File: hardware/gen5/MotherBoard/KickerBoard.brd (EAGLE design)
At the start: 141.6 x 141.1 mm, 154 parts, among them U1 SAM3S4B

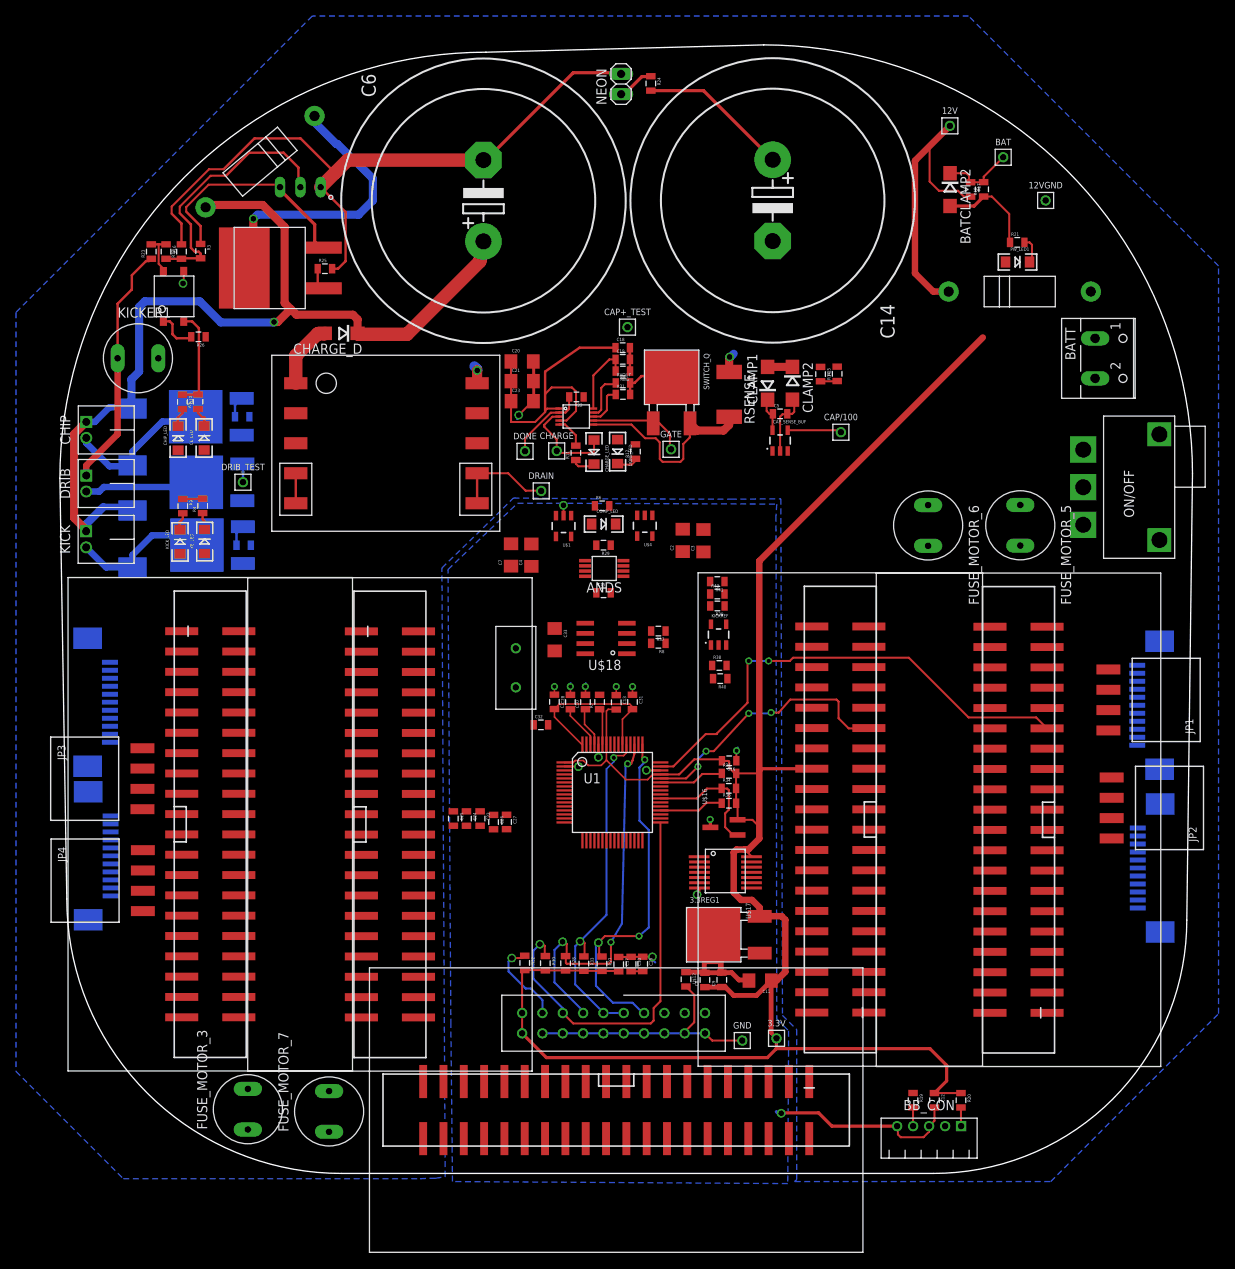
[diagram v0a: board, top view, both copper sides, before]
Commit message: More motherboard work!
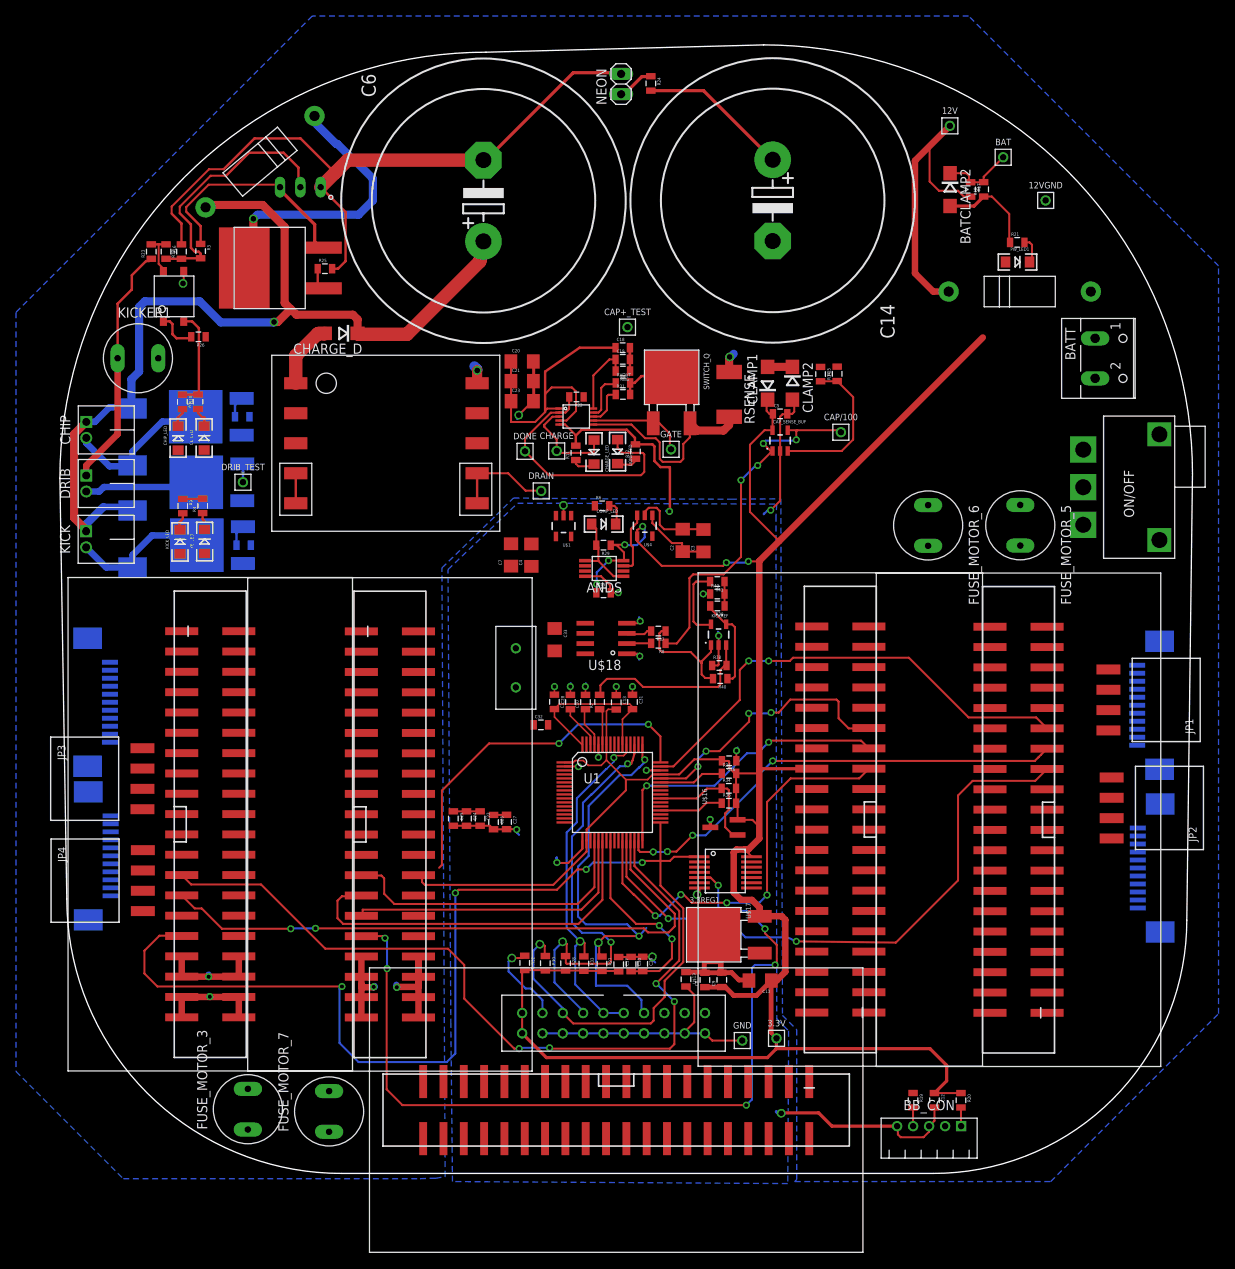
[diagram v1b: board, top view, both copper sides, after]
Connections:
- removed net N$39: MOTOR2.15, MOTOR2.16, MOTOR2.17, MOTOR2.18, U$8.6, U$8.7
- net 12VGND: now also MOTOR1.22, MOTOR1.33, MOTOR1.34, MOTOR2.15, MOTOR2.16, MOTOR2.17, MOTOR2.18, MOTOR2.22, MOTOR2.33, MOTOR2.34, MOTOR3.22, MOTOR3.33, MOTOR3.34, MOTOR4.22, MOTOR4.33, MOTOR4.34, U$10.5, U$11.5, U$8.6, U$8.7, U$9.5
- net GND: no longer MOTOR1.22, MOTOR1.33, MOTOR1.34, MOTOR2.22, MOTOR2.33, MOTOR2.34, MOTOR3.22, MOTOR3.33, MOTOR3.34, MOTOR4.22, MOTOR4.33, MOTOR4.34, U$10.5, U$11.5, U$9.5
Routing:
- net FAULT0: track 0.00 -> 109.2 mm, vias 0 -> 4
- net FAULT3: track 0.00 -> 106.2 mm, vias 0 -> 6
- net DIR0: track 0.00 -> 103.3 mm, vias 0 -> 4
- net 3.3V: track 274.5 -> 370.2 mm, vias 0 -> 6
- net BREN0: track 0.00 -> 76.9 mm, vias 0 -> 2
- net DIR1: track 0.00 -> 75.6 mm, vias 0 -> 2
- net GND: track 123.5 -> 186.3 mm, vias 13 -> 22
- net 12VGND: track 128.2 -> 187.4 mm, vias 5 -> 9
- net BREN1: track 0.00 -> 58.3 mm, vias 0 -> 4
- net DIR2: track 0.00 -> 53.1 mm, vias 0 -> 4
- net BREN3: track 0.00 -> 47.5 mm
- net PWM0: track 0.00 -> 44.4 mm, vias 0 -> 2
- net DIVCAP: track 6.75 -> 47.0 mm, vias 0 -> 4
- net DIR3: track 0.00 -> 38.5 mm
- net PWM3: track 0.00 -> 37.7 mm
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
